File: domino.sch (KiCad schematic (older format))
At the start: 63 parts, among them SW1 SW_PUSH, U1 ProMicro

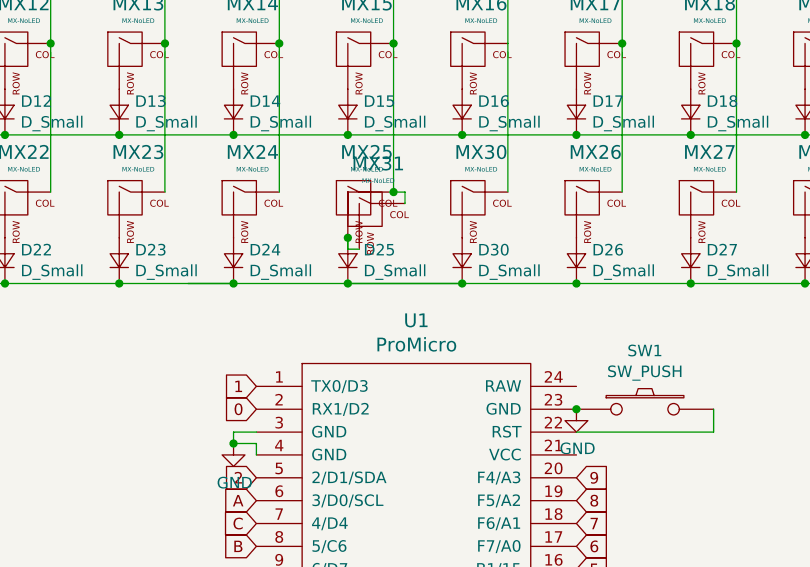
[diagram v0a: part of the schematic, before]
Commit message: uhhh
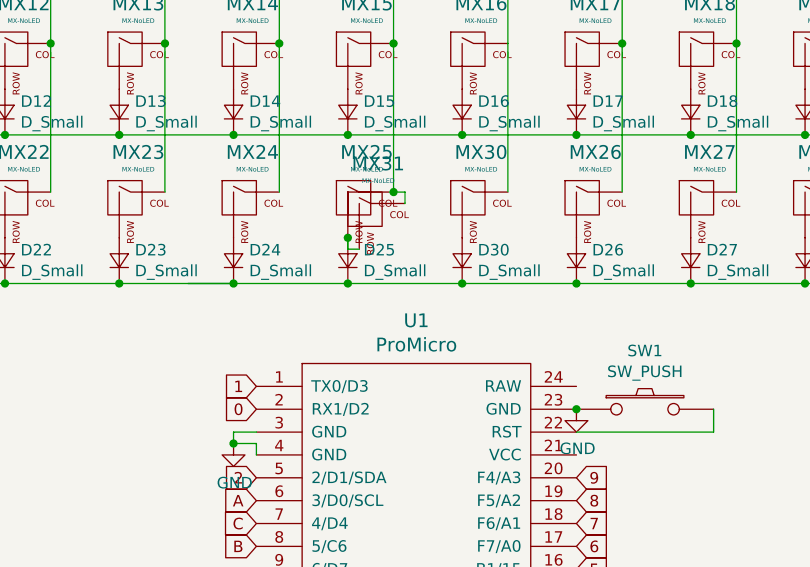
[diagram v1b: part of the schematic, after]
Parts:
- D1, D10, D11, D12, D13, D14, D15, D16, D17, D18, D19, D2, D20, D21, D22, D23, D24, D25, D26, D27, D28, D29, D3, D30, D4, D5, D6, D7, D8, D9: footprint Diode_THT:D_DO-35_SOD27_P7.62mm_Horizontal -> Keebio-Parts:Diode-Hybrid-Back
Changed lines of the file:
@@
 F 0 "D1" V 1696 1682 50  0000 R CNN
 F 1 "D_Small" V 1605 1682 50  0000 R CNN
-F 2 "Diode_THT:D_DO-35_SOD27_P7.62mm_Horizontal" V 1650 1750 50  0001 C CNN
+F 2 "Keebio-Parts:Diode-Hybrid-Back" V 1650 1750 50  0001 C CNN
 F 3 "~" V 1650 1750 50  0001 C CNN
 	1    1650 1750
@@
 F 0 "D11" V 1696 2332 50  0000 R CNN
 F 1 "D_Small" V 1605 2332 50  0000 R CNN
-F 2 "Diode_THT:D_DO-35_SOD27_P7.62mm_Horizontal" V 1650 2400 50  0001 C CNN
+F 2 "Keebio-Parts:Diode-Hybrid-Back" V 1650 2400 50  0001 C CNN
 F 3 "~" V 1650 2400 50  0001 C CNN
 	1    1650 2400
@@
 F 0 "D21" V 1696 2982 50  0000 R CNN
 F 1 "D_Small" V 1605 2982 50  0000 R CNN
-F 2 "Diode_THT:D_DO-35_SOD27_P7.62mm_Horizontal" V 1650 3050 50  0001 C CNN
+F 2 "Keebio-Parts:Diode-Hybrid-Back" V 1650 3050 50  0001 C CNN
 F 3 "~" V 1650 3050 50  0001 C CNN
 	1    1650 3050
@@
 F 0 "D2" V 2196 1682 50  0000 R CNN
 F 1 "D_Small" V 2105 1682 50  0000 R CNN
-F 2 "Diode_THT:D_DO-35_SOD27_P7.62mm_Horizontal" V 2150 1750 50  0001 C CNN
+F 2 "Keebio-Parts:Diode-Hybrid-Back" V 2150 1750 50  0001 C CNN
 F 3 "~" V 2150 1750 50  0001 C CNN
 	1    2150 1750
@@
 F 0 "D12" V 2196 2332 50  0000 R CNN
 F 1 "D_Small" V 2105 2332 50  0000 R CNN
-F 2 "Diode_THT:D_DO-35_SOD27_P7.62mm_Horizontal" V 2150 2400 50  0001 C CNN
+F 2 "Keebio-Parts:Diode-Hybrid-Back" V 2150 2400 50  0001 C CNN
 F 3 "~" V 2150 2400 50  0001 C CNN
 	1    2150 2400
@@
 F 0 "D22" V 2196 2982 50  0000 R CNN
 F 1 "D_Small" V 2105 2982 50  0000 R CNN
-F 2 "Diode_THT:D_DO-35_SOD27_P7.62mm_Horizontal" V 2150 3050 50  0001 C CNN
+F 2 "Keebio-Parts:Diode-Hybrid-Back" V 2150 3050 50  0001 C CNN
 F 3 "~" V 2150 3050 50  0001 C CNN
 	1    2150 3050
@@
 F 0 "D3" V 2696 1682 50  0000 R CNN
 F 1 "D_Small" V 2605 1682 50  0000 R CNN
-F 2 "Diode_THT:D_DO-35_SOD27_P7.62mm_Horizontal" V 2650 1750 50  0001 C CNN
+F 2 "Keebio-Parts:Diode-Hybrid-Back" V 2650 1750 50  0001 C CNN
 F 3 "~" V 2650 1750 50  0001 C CNN
 	1    2650 1750
@@
 F 0 "D13" V 2696 2332 50  0000 R CNN
 F 1 "D_Small" V 2605 2332 50  0000 R CNN
-F 2 "Diode_THT:D_DO-35_SOD27_P7.62mm_Horizontal" V 2650 2400 50  0001 C CNN
+F 2 "Keebio-Parts:Diode-Hybrid-Back" V 2650 2400 50  0001 C CNN
 F 3 "~" V 2650 2400 50  0001 C CNN
 	1    2650 2400
@@
 F 0 "D23" V 2696 2982 50  0000 R CNN
 F 1 "D_Small" V 2605 2982 50  0000 R CNN
-F 2 "Diode_THT:D_DO-35_SOD27_P7.62mm_Horizontal" V 2650 3050 50  0001 C CNN
+F 2 "Keebio-Parts:Diode-Hybrid-Back" V 2650 3050 50  0001 C CNN
 F 3 "~" V 2650 3050 50  0001 C CNN
 	1    2650 3050
@@
 F 0 "D4" V 3196 1682 50  0000 R CNN
 F 1 "D_Small" V 3105 1682 50  0000 R CNN
-F 2 "Diode_THT:D_DO-35_SOD27_P7.62mm_Horizontal" V 3150 1750 50  0001 C CNN
+F 2 "Keebio-Parts:Diode-Hybrid-Back" V 3150 1750 50  0001 C CNN
 F 3 "~" V 3150 1750 50  0001 C CNN
 	1    3150 1750
@@
 F 0 "D14" V 3196 2332 50  0000 R CNN
 F 1 "D_Small" V 3105 2332 50  0000 R CNN
-F 2 "Diode_THT:D_DO-35_SOD27_P7.62mm_Horizontal" V 3150 2400 50  0001 C CNN
+F 2 "Keebio-Parts:Diode-Hybrid-Back" V 3150 2400 50  0001 C CNN
 F 3 "~" V 3150 2400 50  0001 C CNN
 	1    3150 2400
@@
 F 0 "D24" V 3196 2982 50  0000 R CNN
 F 1 "D_Small" V 3105 2982 50  0000 R CNN
-F 2 "Diode_THT:D_DO-35_SOD27_P7.62mm_Horizontal" V 3150 3050 50  0001 C CNN
+F 2 "Keebio-Parts:Diode-Hybrid-Back" V 3150 3050 50  0001 C CNN
 F 3 "~" V 3150 3050 50  0001 C CNN
 	1    3150 3050
@@
 F 0 "D5" V 3696 1682 50  0000 R CNN
 F 1 "D_Small" V 3605 1682 50  0000 R CNN
-F 2 "Diode_THT:D_DO-35_SOD27_P7.62mm_Horizontal" V 3650 1750 50  0001 C CNN
+F 2 "Keebio-Parts:Diode-Hybrid-Back" V 3650 1750 50  0001 C CNN
 F 3 "~" V 3650 1750 50  0001 C CNN
 	1    3650 1750
@@
 F 0 "D15" V 3696 2332 50  0000 R CNN
 F 1 "D_Small" V 3605 2332 50  0000 R CNN
-F 2 "Diode_THT:D_DO-35_SOD27_P7.62mm_Horizontal" V 3650 2400 50  0001 C CNN
+F 2 "Keebio-Parts:Diode-Hybrid-Back" V 3650 2400 50  0001 C CNN
 F 3 "~" V 3650 2400 50  0001 C CNN
 	1    3650 2400
@@
 F 0 "D6" V 4196 1682 50  0000 R CNN
 F 1 "D_Small" V 4105 1682 50  0000 R CNN
-F 2 "Diode_THT:D_DO-35_SOD27_P7.62mm_Horizontal" V 4150 1750 50  0001 C CNN
+F 2 "Keebio-Parts:Diode-Hybrid-Back" V 4150 1750 50  0001 C CNN
 F 3 "~" V 4150 1750 50  0001 C CNN
 	1    4150 1750
@@
 F 0 "D16" V 4196 2332 50  0000 R CNN
 F 1 "D_Small" V 4105 2332 50  0000 R CNN
-F 2 "Diode_THT:D_DO-35_SOD27_P7.62mm_Horizontal" V 4150 2400 50  0001 C CNN
+F 2 "Keebio-Parts:Diode-Hybrid-Back" V 4150 2400 50  0001 C CNN
 F 3 "~" V 4150 2400 50  0001 C CNN
 	1    4150 2400
@@
 F 0 "D25" V 3696 2982 50  0000 R CNN
 F 1 "D_Small" V 3605 2982 50  0000 R CNN
-F 2 "Diode_THT:D_DO-35_SOD27_P7.62mm_Horizontal" V 3650 3050 50  0001 C CNN
+F 2 "Keebio-Parts:Diode-Hybrid-Back" V 3650 3050 50  0001 C CNN
 F 3 "~" V 3650 3050 50  0001 C CNN
 	1    3650 3050
@@
 F 0 "D7" V 4696 1682 50  0000 R CNN
 F 1 "D_Small" V 4605 1682 50  0000 R CNN
-F 2 "Diode_THT:D_DO-35_SOD27_P7.62mm_Horizontal" V 4650 1750 50  0001 C CNN
+F 2 "Keebio-Parts:Diode-Hybrid-Back" V 4650 1750 50  0001 C CNN
 F 3 "~" V 4650 1750 50  0001 C CNN
 	1    4650 1750
@@
 F 0 "D17" V 4696 2332 50  0000 R CNN
 F 1 "D_Small" V 4605 2332 50  0000 R CNN
-F 2 "Diode_THT:D_DO-35_SOD27_P7.62mm_Horizontal" V 4650 2400 50  0001 C CNN
+F 2 "Keebio-Parts:Diode-Hybrid-Back" V 4650 2400 50  0001 C CNN
 F 3 "~" V 4650 2400 50  0001 C CNN
 	1    4650 2400
@@
 F 0 "D26" V 4696 2982 50  0000 R CNN
 F 1 "D_Small" V 4605 2982 50  0000 R CNN
-F 2 "Diode_THT:D_DO-35_SOD27_P7.62mm_Horizontal" V 4650 3050 50  0001 C CNN
+F 2 "Keebio-Parts:Diode-Hybrid-Back" V 4650 3050 50  0001 C CNN
 F 3 "~" V 4650 3050 50  0001 C CNN
 	1    4650 3050
@@
 F 0 "D8" V 5196 1682 50  0000 R CNN
 F 1 "D_Small" V 5105 1682 50  0000 R CNN
-F 2 "Diode_THT:D_DO-35_SOD27_P7.62mm_Horizontal" V 5150 1750 50  0001 C CNN
+F 2 "Keebio-Parts:Diode-Hybrid-Back" V 5150 1750 50  0001 C CNN
 F 3 "~" V 5150 1750 50  0001 C CNN
 	1    5150 1750
@@
 F 0 "D18" V 5196 2332 50  0000 R CNN
 F 1 "D_Small" V 5105 2332 50  0000 R CNN
-F 2 "Diode_THT:D_DO-35_SOD27_P7.62mm_Horizontal" V 5150 2400 50  0001 C CNN
+F 2 "Keebio-Parts:Diode-Hybrid-Back" V 5150 2400 50  0001 C CNN
 F 3 "~" V 5150 2400 50  0001 C CNN
 	1    5150 2400
@@
 F 0 "D27" V 5196 2982 50  0000 R CNN
 F 1 "D_Small" V 5105 2982 50  0000 R CNN
-F 2 "Diode_THT:D_DO-35_SOD27_P7.62mm_Horizontal" V 5150 3050 50  0001 C CNN
+F 2 "Keebio-Parts:Diode-Hybrid-Back" V 5150 3050 50  0001 C CNN
 F 3 "~" V 5150 3050 50  0001 C CNN
 	1    5150 3050
@@
 F 0 "D9" V 5696 1682 50  0000 R CNN
 F 1 "D_Small" V 5605 1682 50  0000 R CNN
-F 2 "Diode_THT:D_DO-35_SOD27_P7.62mm_Horizontal" V 5650 1750 50  0001 C CNN
+F 2 "Keebio-Parts:Diode-Hybrid-Back" V 5650 1750 50  0001 C CNN
 F 3 "~" V 5650 1750 50  0001 C CNN
 	1    5650 1750
@@
 F 0 "D19" V 5696 2332 50  0000 R CNN
 F 1 "D_Small" V 5605 2332 50  0000 R CNN
-F 2 "Diode_THT:D_DO-35_SOD27_P7.62mm_Horizontal" V 5650 2400 50  0001 C CNN
+F 2 "Keebio-Parts:Diode-Hybrid-Back" V 5650 2400 50  0001 C CNN
 F 3 "~" V 5650 2400 50  0001 C CNN
 	1    5650 2400
@@
 F 0 "D28" V 5696 2982 50  0000 R CNN
 F 1 "D_Small" V 5605 2982 50  0000 R CNN
-F 2 "Diode_THT:D_DO-35_SOD27_P7.62mm_Horizontal" V 5650 3050 50  0001 C CNN
+F 2 "Keebio-Parts:Diode-Hybrid-Back" V 5650 3050 50  0001 C CNN
 F 3 "~" V 5650 3050 50  0001 C CNN
 	1    5650 3050
@@
 F 0 "D10" V 6196 1682 50  0000 R CNN
 F 1 "D_Small" V 6105 1682 50  0000 R CNN
-F 2 "Diode_THT:D_DO-35_SOD27_P7.62mm_Horizontal" V 6150 1750 50  0001 C CNN
+F 2 "Keebio-Parts:Diode-Hybrid-Back" V 6150 1750 50  0001 C CNN
 F 3 "~" V 6150 1750 50  0001 C CNN
 	1    6150 1750
@@
 F 0 "D20" V 6196 2332 50  0000 R CNN
 F 1 "D_Small" V 6105 2332 50  0000 R CNN
-F 2 "Diode_THT:D_DO-35_SOD27_P7.62mm_Horizontal" V 6150 2400 50  0001 C CNN
+F 2 "Keebio-Parts:Diode-Hybrid-Back" V 6150 2400 50  0001 C CNN
 F 3 "~" V 6150 2400 50  0001 C CNN
 	1    6150 2400
@@
 F 0 "D29" V 6196 2982 50  0000 R CNN
 F 1 "D_Small" V 6105 2982 50  0000 R CNN
-F 2 "Diode_THT:D_DO-35_SOD27_P7.62mm_Horizontal" V 6150 3050 50  0001 C CNN
+F 2 "Keebio-Parts:Diode-Hybrid-Back" V 6150 3050 50  0001 C CNN
 F 3 "~" V 6150 3050 50  0001 C CNN
 	1    6150 3050
@@
 F 0 "D30" V 4196 2982 50  0000 R CNN
 F 1 "D_Small" V 4105 2982 50  0000 R CNN
-F 2 "Diode_THT:D_DO-35_SOD27_P7.62mm_Horizontal" V 4150 3050 50  0001 C CNN
+F 2 "Keebio-Parts:Diode-Hybrid-Back" V 4150 3050 50  0001 C CNN
 F 3 "~" V 4150 3050 50  0001 C CNN
 	1    4150 3050
@@
 Wire Wire Line
 	4350 2100 4350 2750
-Wire Wire Line
-	3650 3150 4150 3150
 Connection ~ 4150 3150
 Wire Wire Line
